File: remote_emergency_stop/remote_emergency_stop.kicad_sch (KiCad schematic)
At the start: 13 parts, among them J1 Conn_01x02, U1 MOUDLE-SEEEDUINO-XIAO-ESP32C3

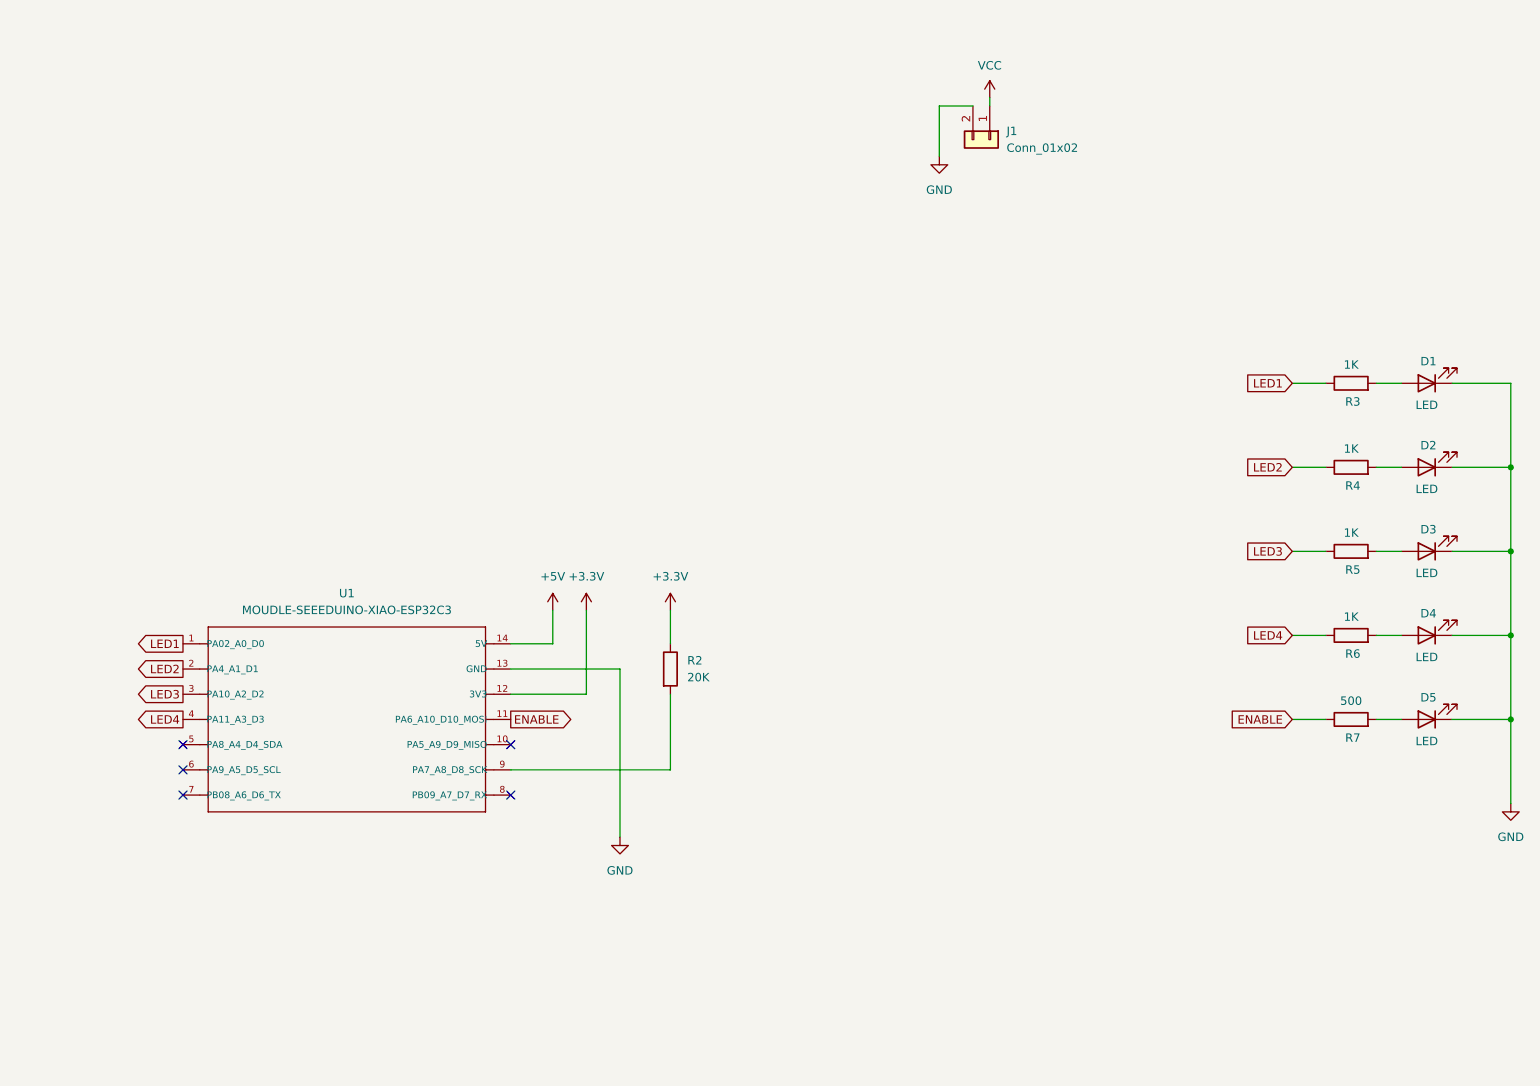
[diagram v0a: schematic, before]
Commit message: こりゃだめだ、ユーザーインタフェイスが整ってない。
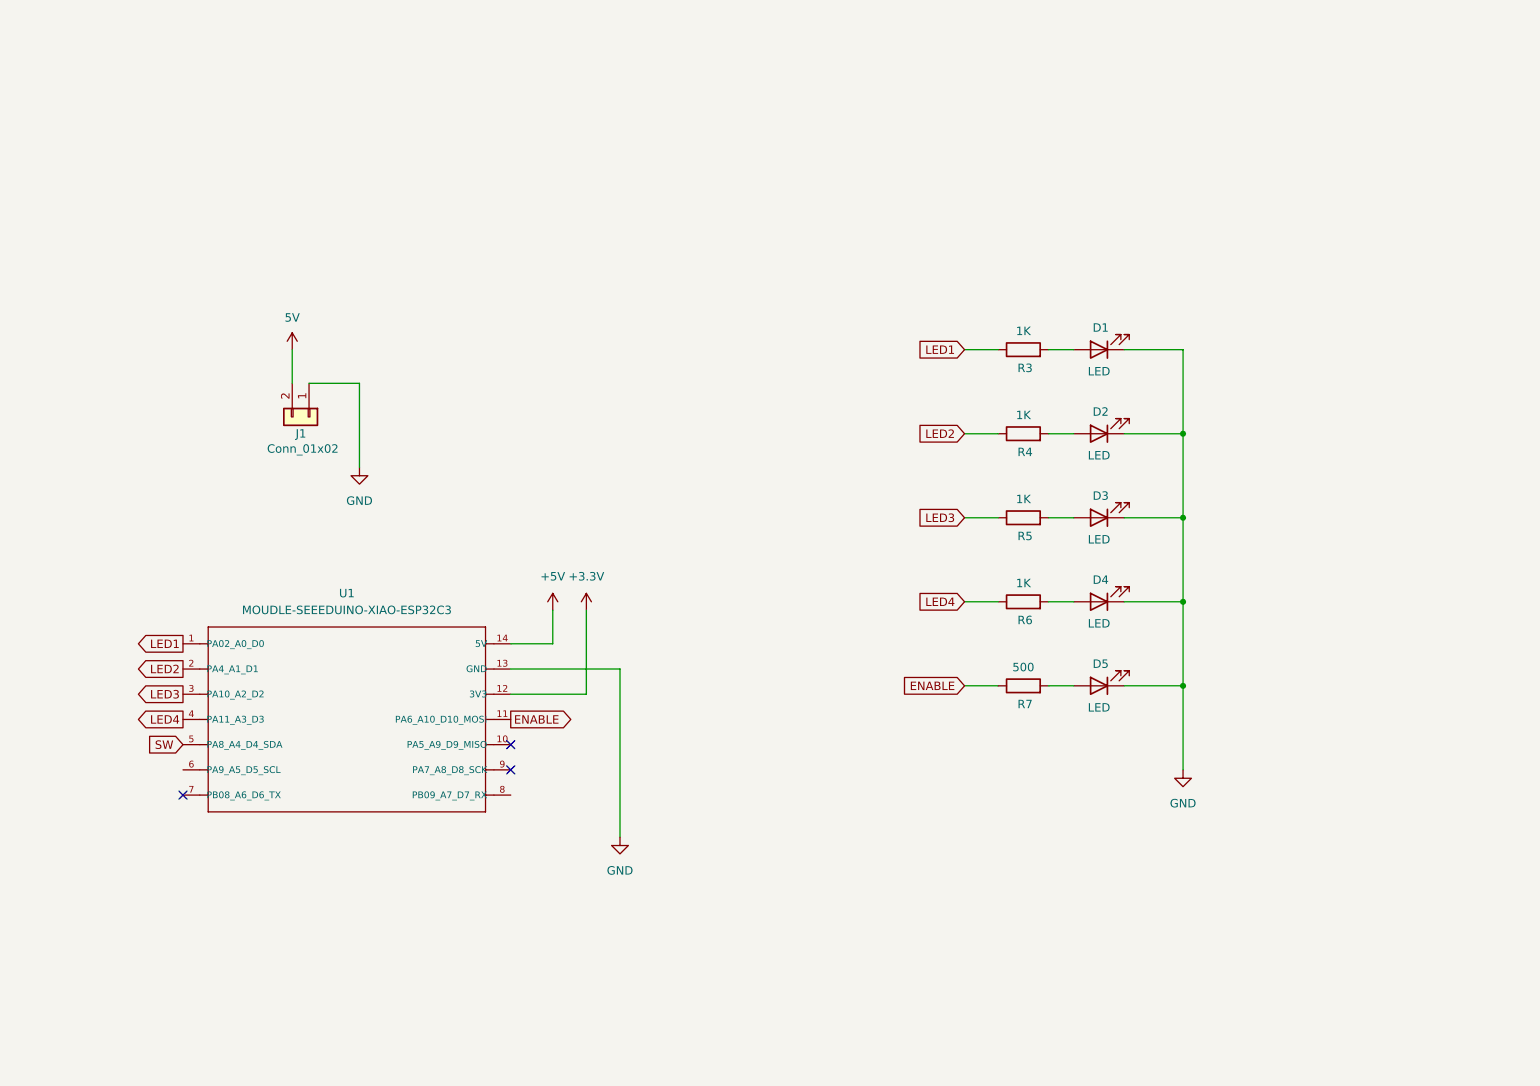
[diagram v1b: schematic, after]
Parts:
- removed R2: 20K, symbol Device:R
- D1, D2, D3, D4, D5: footprint (none) -> LED_SMD:LED_0603_1608Metric_Pad1.05x0.95mm_HandSolder
- J1: footprint Connector_AMASS:AMASS_XT30U-M_1x02_P5.0mm_Vertical -> Connector_JST:JST_XH_S2B-XH-A_1x02_P2.50mm_Horizontal
- R3, R4, R5, R6, R7: footprint (none) -> Resistor_SMD:R_0603_1608Metric_Pad0.98x0.95mm_HandSolder
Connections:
- net VCC is gone; now on net GND: J1.1 (Pin_1)
- net GND: no longer J1.2 (Pin_2)
- net SW: now reaches U1.5 (PA8_A4_D4_SDA)
- new net 5V: J1.2 (Pin_2)
- no-connect marks 5 -> 3
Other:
- moved on the sheet: D1, D2, D3, D4, D5, J1, R3, R4, R5, R6, R7

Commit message: 遠隔非常停止は回路だけ完成した気がする
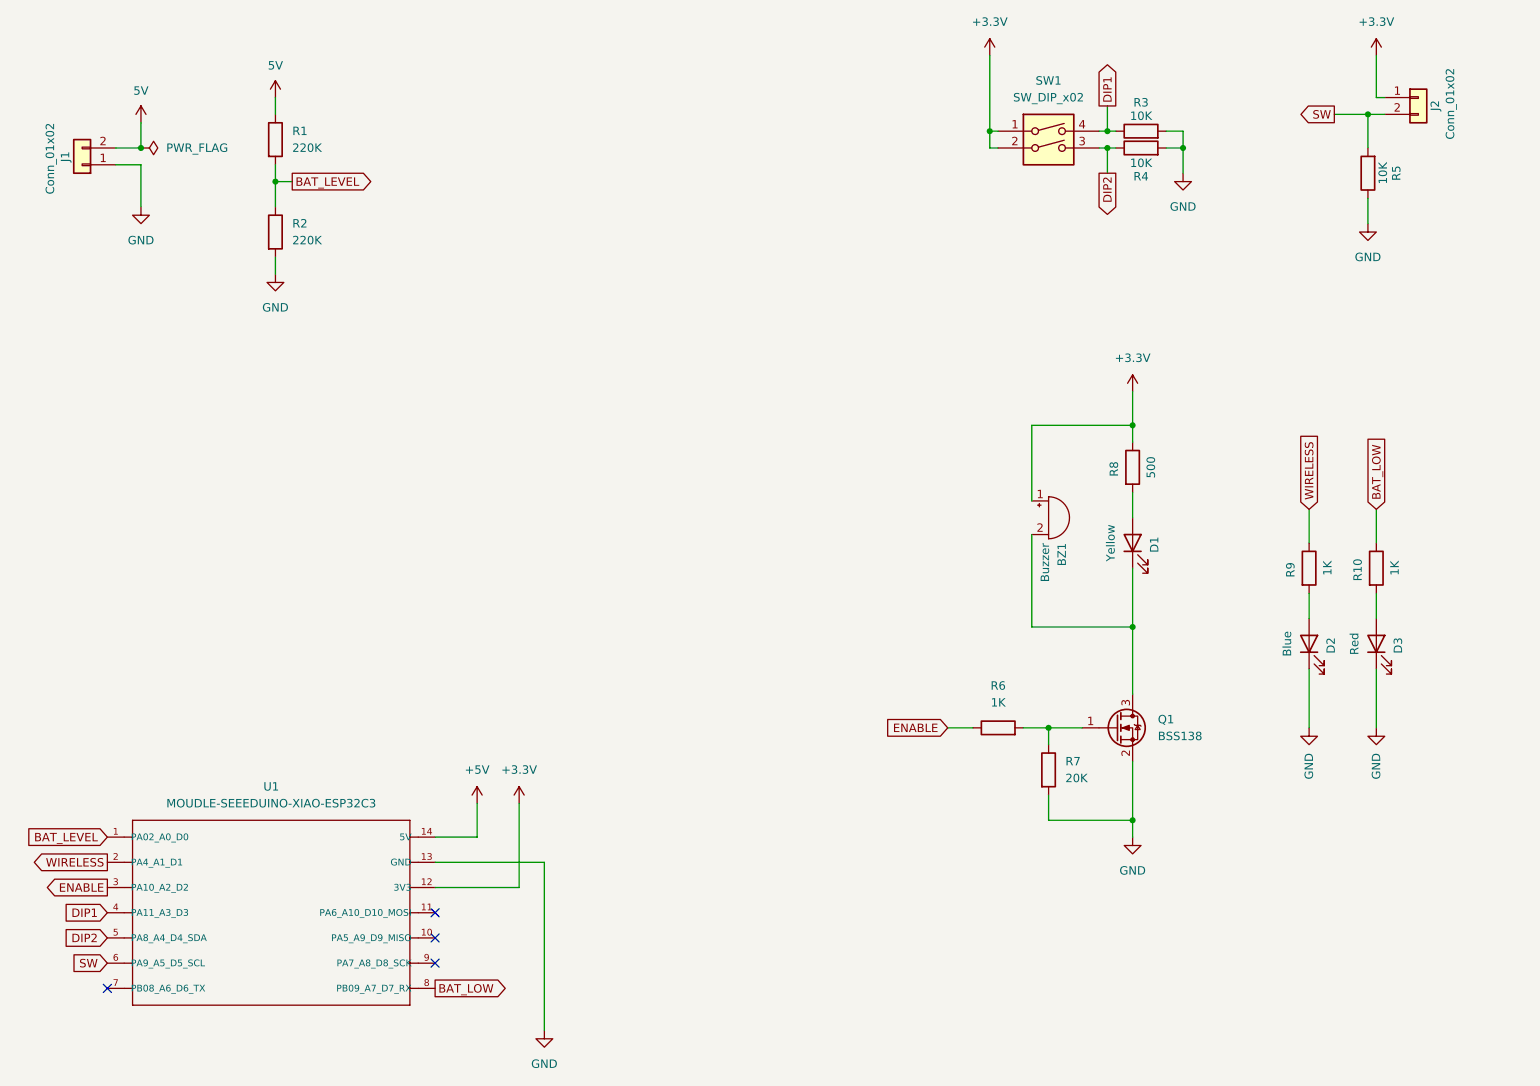
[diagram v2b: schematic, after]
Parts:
- removed D2, D5: LED, LED_SMD:LED_0603_1608Metric_Pad1.05x0.95mm_HandSolder, symbol Device:LED
- added BZ1: Buzzer, Buzzer_Beeper:Buzzer_12x9.5RM7.6, symbol Device:Buzzer
- added J2: Conn_01x02, Connector_JST:JST_XH_S2B-XH-A_1x02_P2.50mm_Horizontal, symbol Connector_Generic:Conn_01x02
- added Q1: BSS138, Package_TO_SOT_SMD:SOT-23, symbol Transistor_FET:AO3400A
- added R1, R2: 220K, Resistor_SMD:R_0603_1608Metric, symbol Device:R
- added R10, R6: 1K, Resistor_SMD:R_0603_1608Metric, symbol Device:R
- added R8: 500, Resistor_SMD:R_0603_1608Metric, symbol Device:R
- added SW1: SW_DIP_x02, Button_Switch_SMD:SW_DIP_SPSTx02_Slide_Omron_A6H-2101_W6.15mm_P1.27mm, symbol Switch:SW_DIP_x02
- D1: value LED -> Yellow
- D2: renamed from D4; value LED -> Blue
- D3: value LED -> Red
- R3, R4, R5: value 1K -> 10K; footprint Resistor_SMD:R_0603_1608Metric_Pad0.98x0.95mm_HandSolder -> Resistor_SMD:R_0603_1608Metric
- R7: value 500 -> 20K; footprint Resistor_SMD:R_0603_1608Metric_Pad0.98x0.95mm_HandSolder -> Resistor_SMD:R_0603_1608Metric
- R9: renamed from R6; footprint Resistor_SMD:R_0603_1608Metric_Pad0.98x0.95mm_HandSolder -> Resistor_SMD:R_0603_1608Metric
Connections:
- net +3.3V: now also BZ1.1 (+), J2.1 (Pin_1), R8.1, SW1.1, SW1.2
- net 5V: now also R1.1
- net ENABLE: now also U1.3 (PA10_A2_D2), R6.1; no longer R7.1, U1.11 (PA6_A10_D10_MOSI)
- net GND: now also R3.2, R4.2, R5.1, R7.2, Q1.2 (S), R2.2; no longer D1.1 (K)
- net SW: now also R5.2, U1.6 (PA9_A5_D5_SCL), J2.2 (Pin_2); no longer U1.5 (PA8_A4_D4_SDA)
- net at D1.2 (A): now also R8.2; no longer R3.2
- net at D3.2 (A): now also R10.2; no longer R5.2
- net BAT_LOW: now reaches U1.8 (PB09_A7_D7_RX)
- net BAT_LOW: now also R10.1
- net LED1 renamed BAT_LEVEL
- net BAT_LEVEL: now also R1.2, R2.1; no longer R3.1
- net LED2 renamed DIP2
- net DIP2: now also U1.5 (PA8_A4_D4_SDA), SW1.3; no longer U1.2 (PA4_A1_D1)
- removed net LED3: R5.1, U1.3 (PA10_A2_D2)
- net LED4 renamed DIP1
- net DIP1: now also R3.1, SW1.4; no longer R9.1
- new net: BZ1.2 (-), D1.1 (K), Q1.3 (D)
- new net: Q1.1 (G), R6.2, R7.1
- new net WIRELESS: R9.1, U1.2 (PA4_A1_D1)
- no-connect marks 3 -> 4
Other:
- moved on the sheet: D2, J1, R9, U1
